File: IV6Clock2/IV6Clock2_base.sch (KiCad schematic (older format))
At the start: 40 parts, among them J1 DC005, J2 Debug, J3 Conn_01x04, J4 Conn_01x04, J5 Conn_01x04, J6 Conn_01x01, SW1 <, SW2 v, SW3 >, U1 ATmega328P-PU, U2 DS3231M, U3 TLV62568DBV, U4 AP3012KTR, U5 DS3232M

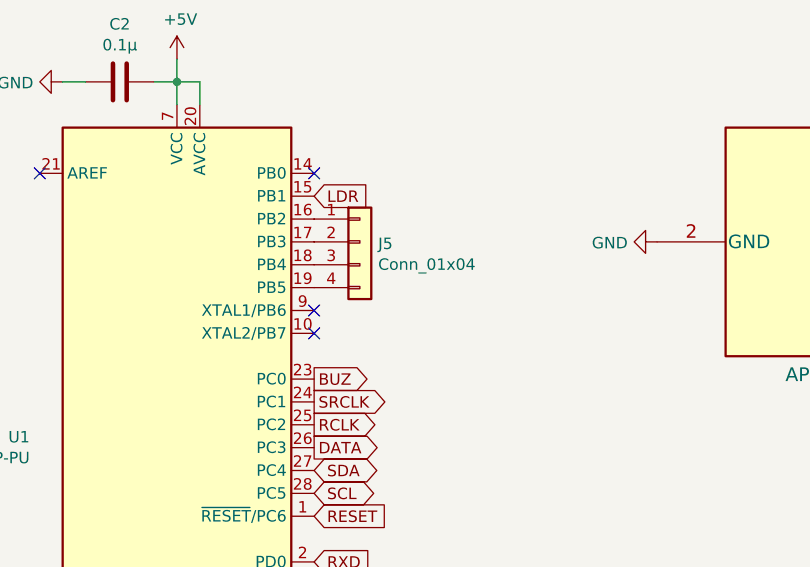
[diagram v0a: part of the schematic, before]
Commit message: Fixed wrong pin i/o on base board
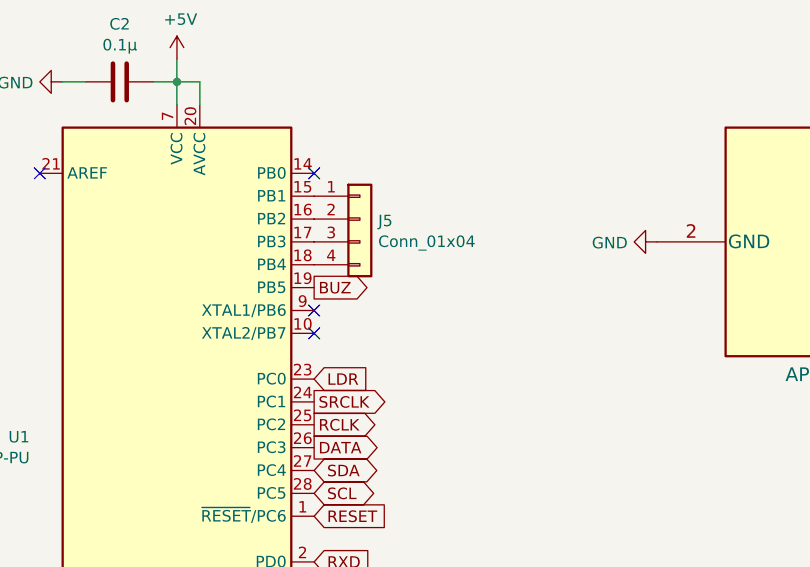
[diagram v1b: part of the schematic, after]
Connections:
- net BUZ: now also U1.19 (PB5); no longer U1.23 (PC0)
- net LDR: now also U1.23 (PC0); no longer U1.15 (PB1)
- net at J5.1 (Pin_1): now also U1.15 (PB1); no longer U1.16 (PB2)
- net at J5.2 (Pin_2): now also U1.16 (PB2); no longer U1.17 (PB3)
- net at J5.3 (Pin_3): now also U1.17 (PB3); no longer U1.18 (PB4)
- net at J5.4 (Pin_4): now also U1.18 (PB4); no longer U1.19 (PB5)
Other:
- moved on the sheet: J5
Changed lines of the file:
@@
 Text GLabel 2200 4000 2    50   BiDi ~ 0
 SCL
-Text GLabel 2200 2700 2    50   Input ~ 0
+Text GLabel 2200 3500 2    50   Input ~ 0
 LDR
-Text GLabel 2200 3500 2    50   Output ~ 0
+Text GLabel 2200 3100 2    50   Output ~ 0
 BUZ
 $Comp
@@
 L Connector_Generic:Conn_01x04 J5
 U 1 1 5F22E5EE
-P 2400 2900
-F 0 "J5" H 2480 2892 50  0000 L CNN
-F 1 "Conn_01x04" H 2480 2801 50  0000 L CNN
-F 2 "Connector_PinSocket_2.54mm:PinSocket_1x04_P2.54mm_Vertical" H 2400 2900 50  0001 C CNN
-F 3 "~" H 2400 2900 50  0001 C CNN
-	1    2400 2900
-	1    0    0    -1
-$EndComp
+P 2400 2800
+F 0 "J5" H 2480 2792 50  0000 L CNN
+F 1 "Conn_01x04" H 2480 2701 50  0000 L CNN
+F 2 "Connector_PinSocket_2.54mm:PinSocket_1x04_P2.54mm_Vertical" H 2400 2800 50  0001 C CNN
+F 3 "~" H 2400 2800 50  0001 C CNN
+	1    2400 2800
+	1    0    0    -1
+$EndComp
